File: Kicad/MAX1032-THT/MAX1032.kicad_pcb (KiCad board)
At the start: 2 copper layers, 24.6 x 16.2 mm, 7 parts, among them U1 MAX1032BEUG_

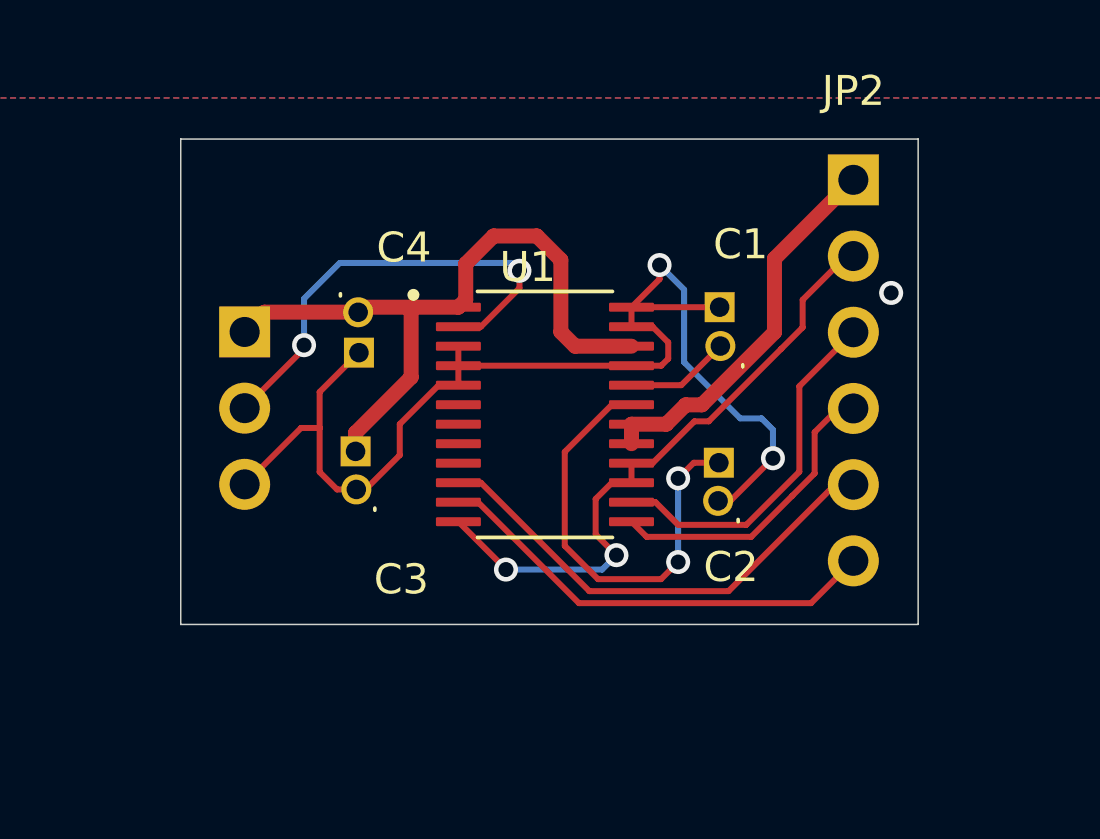
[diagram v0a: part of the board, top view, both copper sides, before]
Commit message: Add files via upload
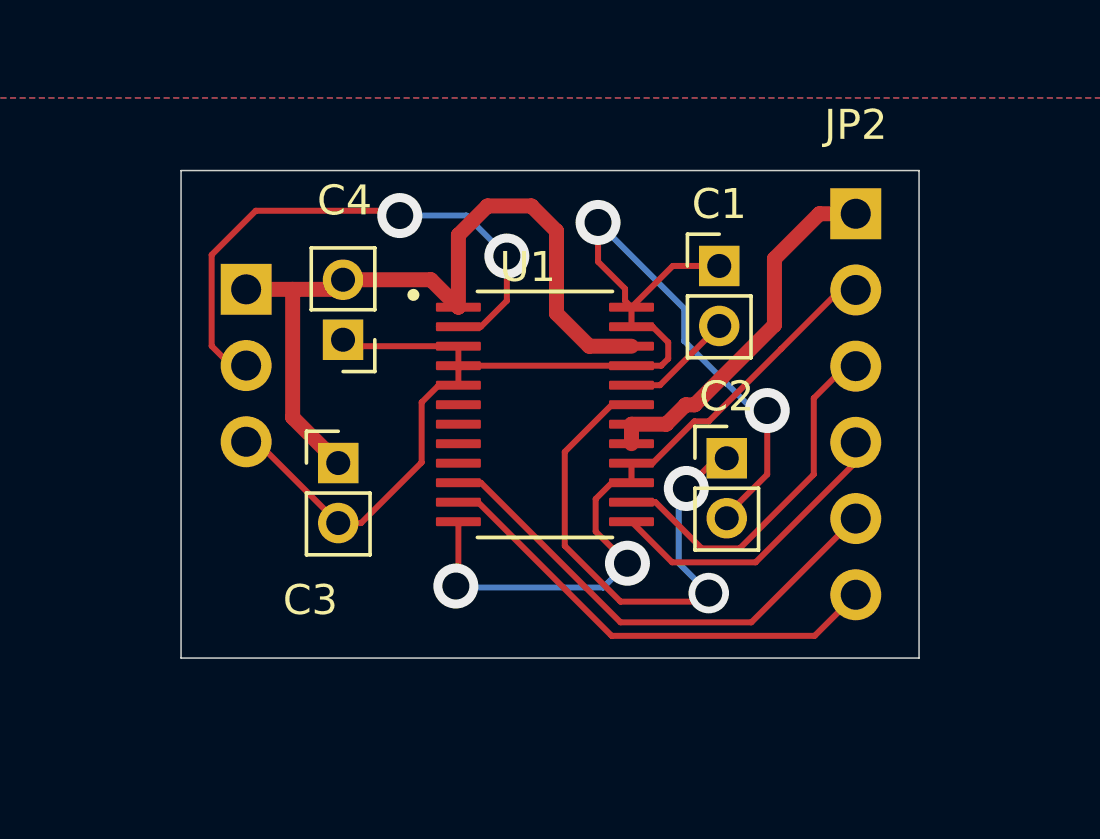
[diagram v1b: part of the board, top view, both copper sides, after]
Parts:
- C1, C2, C3, C4: footprint Connector_PinHeader_1.27mm:PinHeader_1x02_P1.27mm_Horizontal -> Connector_PinHeader_2.00mm:PinHeader_1x02_P2.00mm_Vertical
- moved C1 1.44 mm to (104.6, 90.6)
- moved JP1 1.42 mm to (88.8, 91.4)
- moved JP2 1.13 mm to (109.2, 88.9)
- moved C3 0.87 mm to (91.9, 97.2)
- moved C4 0.56 mm to (92.1, 93.1)
- moved C2 0.16 mm to (104.8, 97.0)
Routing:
- net GND: track 41.3 -> 47.0 mm, vias 3 -> 2
- net /CH0: track 15.4 -> 19.7 mm
- net /AVDD: track 23.6 -> 26.1 mm
- net Net-(U1-REFCAP): track 14.8 -> 17.1 mm
- net /DGND: track 21.2 -> 22.8 mm
- net /DVDD: track 12.9 -> 12.3 mm
- net /DIN: track 15.1 -> 15.7 mm

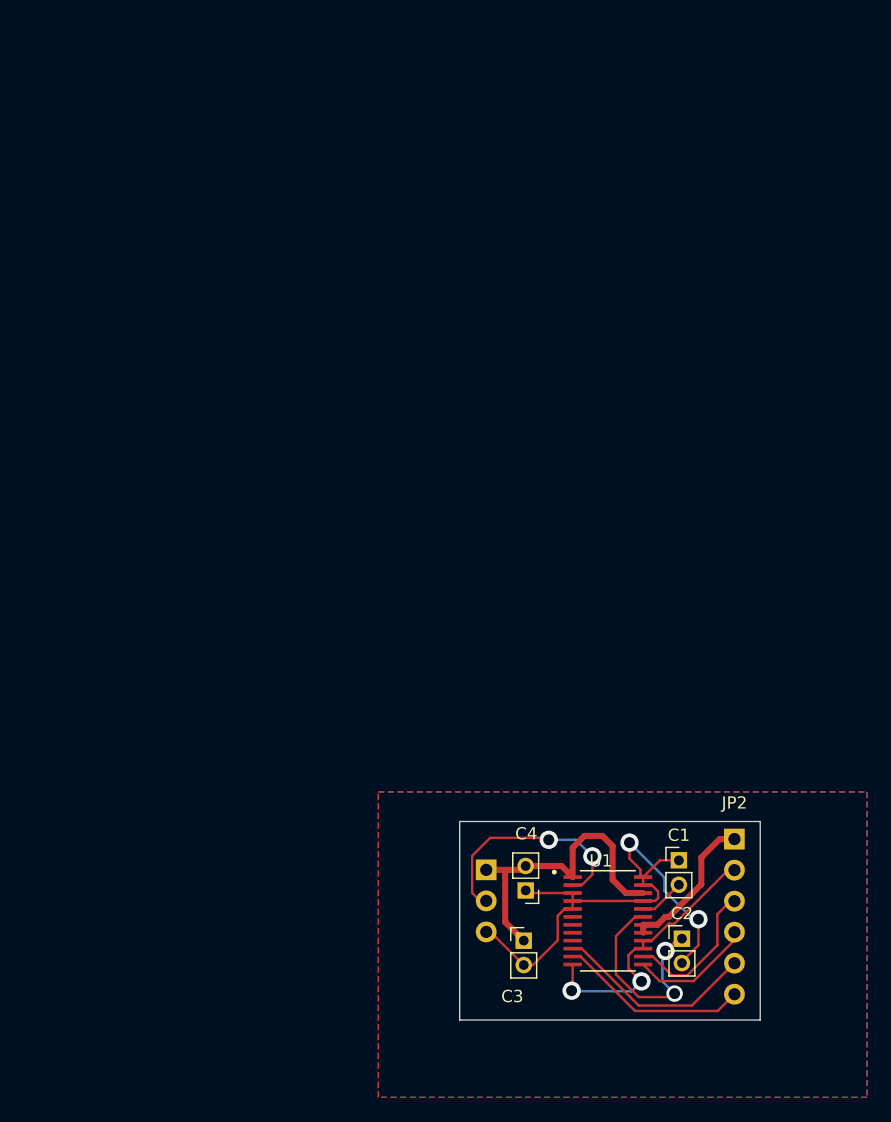
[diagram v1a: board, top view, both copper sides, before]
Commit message: Add files via upload
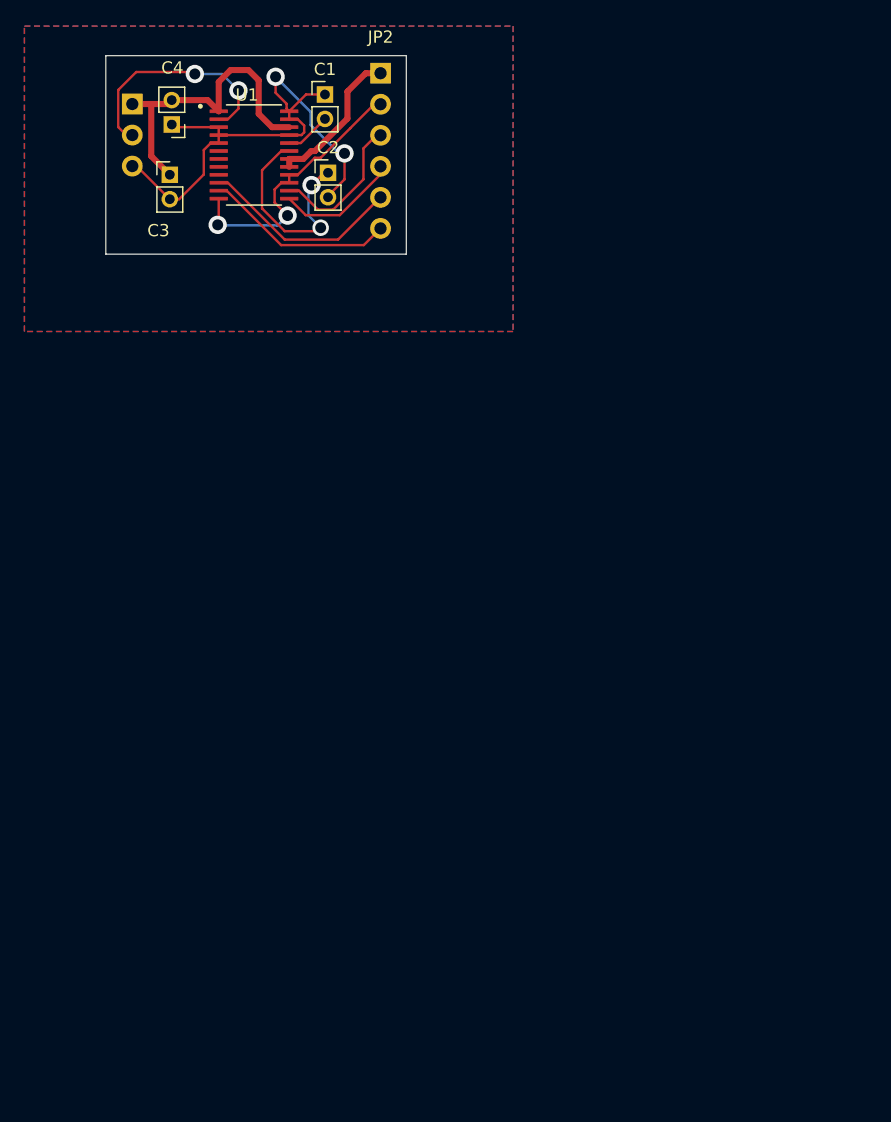
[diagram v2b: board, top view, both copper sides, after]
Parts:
- moved C1 69.1 mm to (75.6, 27.9)
- moved C2 69.1 mm to (75.9, 34.3)
- moved C3 69.1 mm to (62.9, 34.5)
- moved C4 69.1 mm to (63.1, 30.4)
- moved JP1 69.1 mm to (59.9, 28.7)
- moved JP2 69.1 mm to (80.2, 26.2)
- moved U1 69.1 mm to (69.8, 32.9)
